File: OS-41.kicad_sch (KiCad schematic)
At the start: 70 parts, among them J1 Conn_01x02_Pin, J2 Conn_01x02_Pin, J3 Conn_01x02_Pin, J4 Conn_Coaxial, J5 Conn_01x02_Pin, J6 Conn_01x04_Pin, J7 Conn_01x09_Pin, J8 Conn_01x02_Pin, J9 Conn_01x02_Pin, U1 GPS1003, U2 SI4432-B1-FMR, U3 MCP1640x-xCHY, U4 ATGM336H-5N31, U5 DS18B20, U6 BMP390L, U7 STM32F411CEUx, X1 SMD-3225_4P 30.000MHZ 10PF, Y1 Crystal_GND24, Y2 Crystal

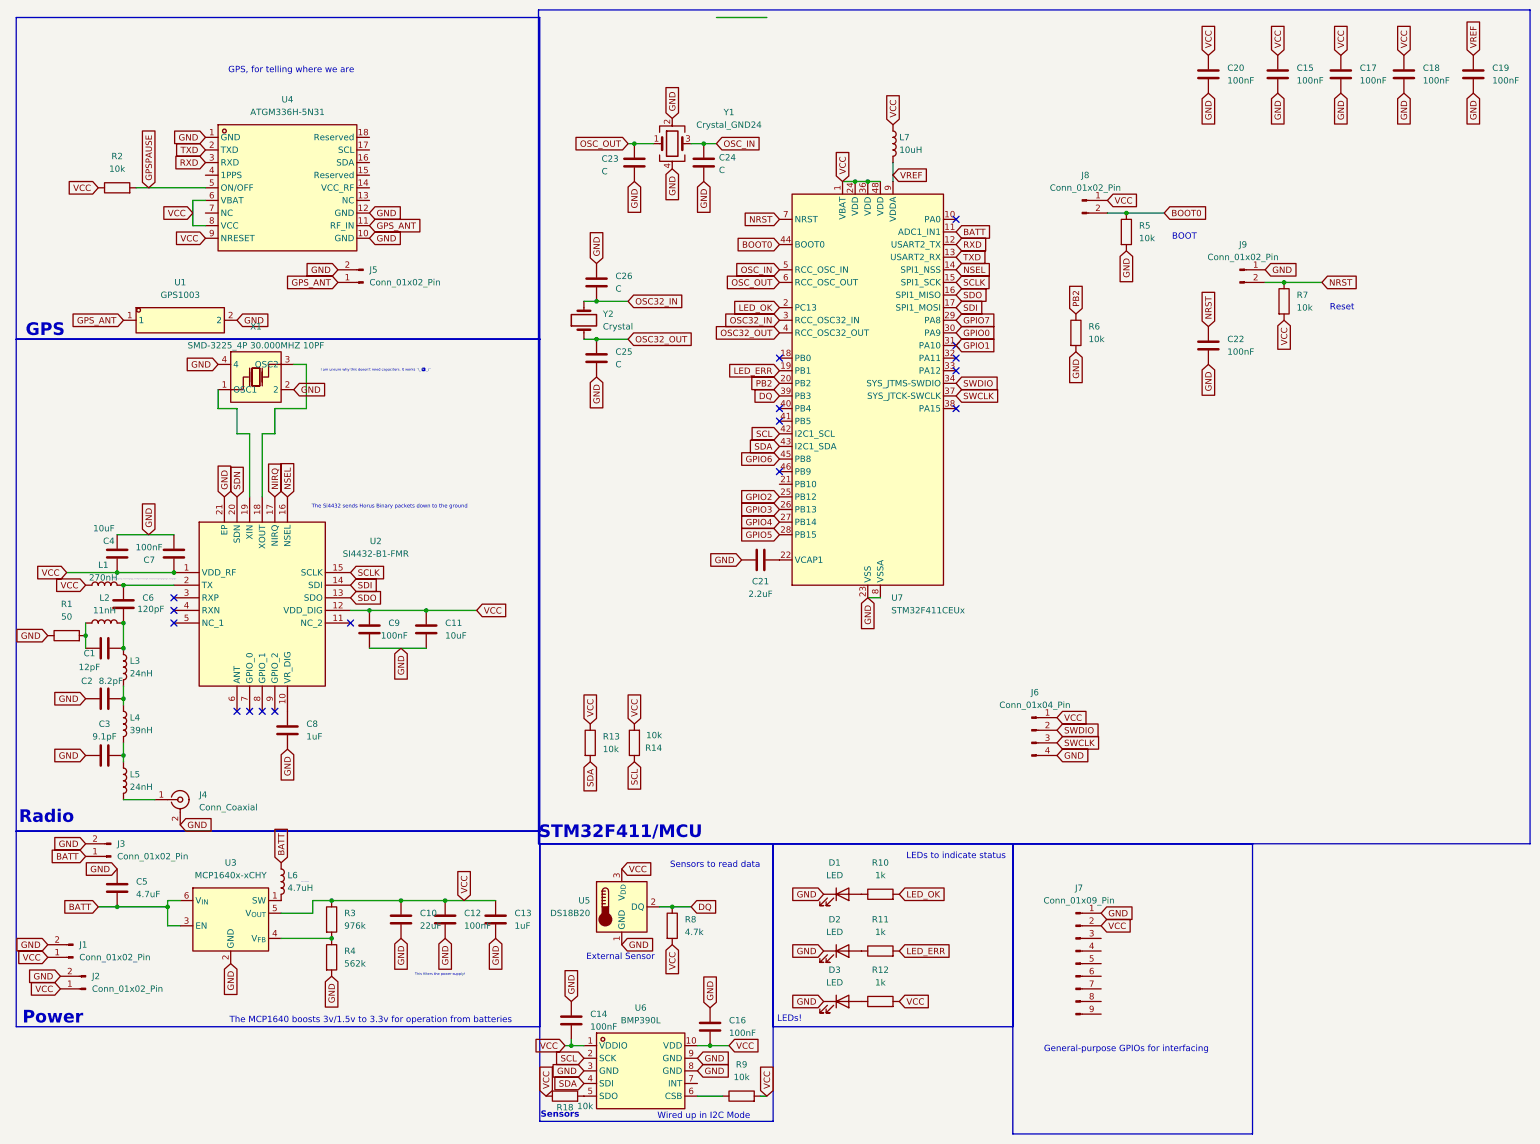
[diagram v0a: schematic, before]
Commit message: Progress
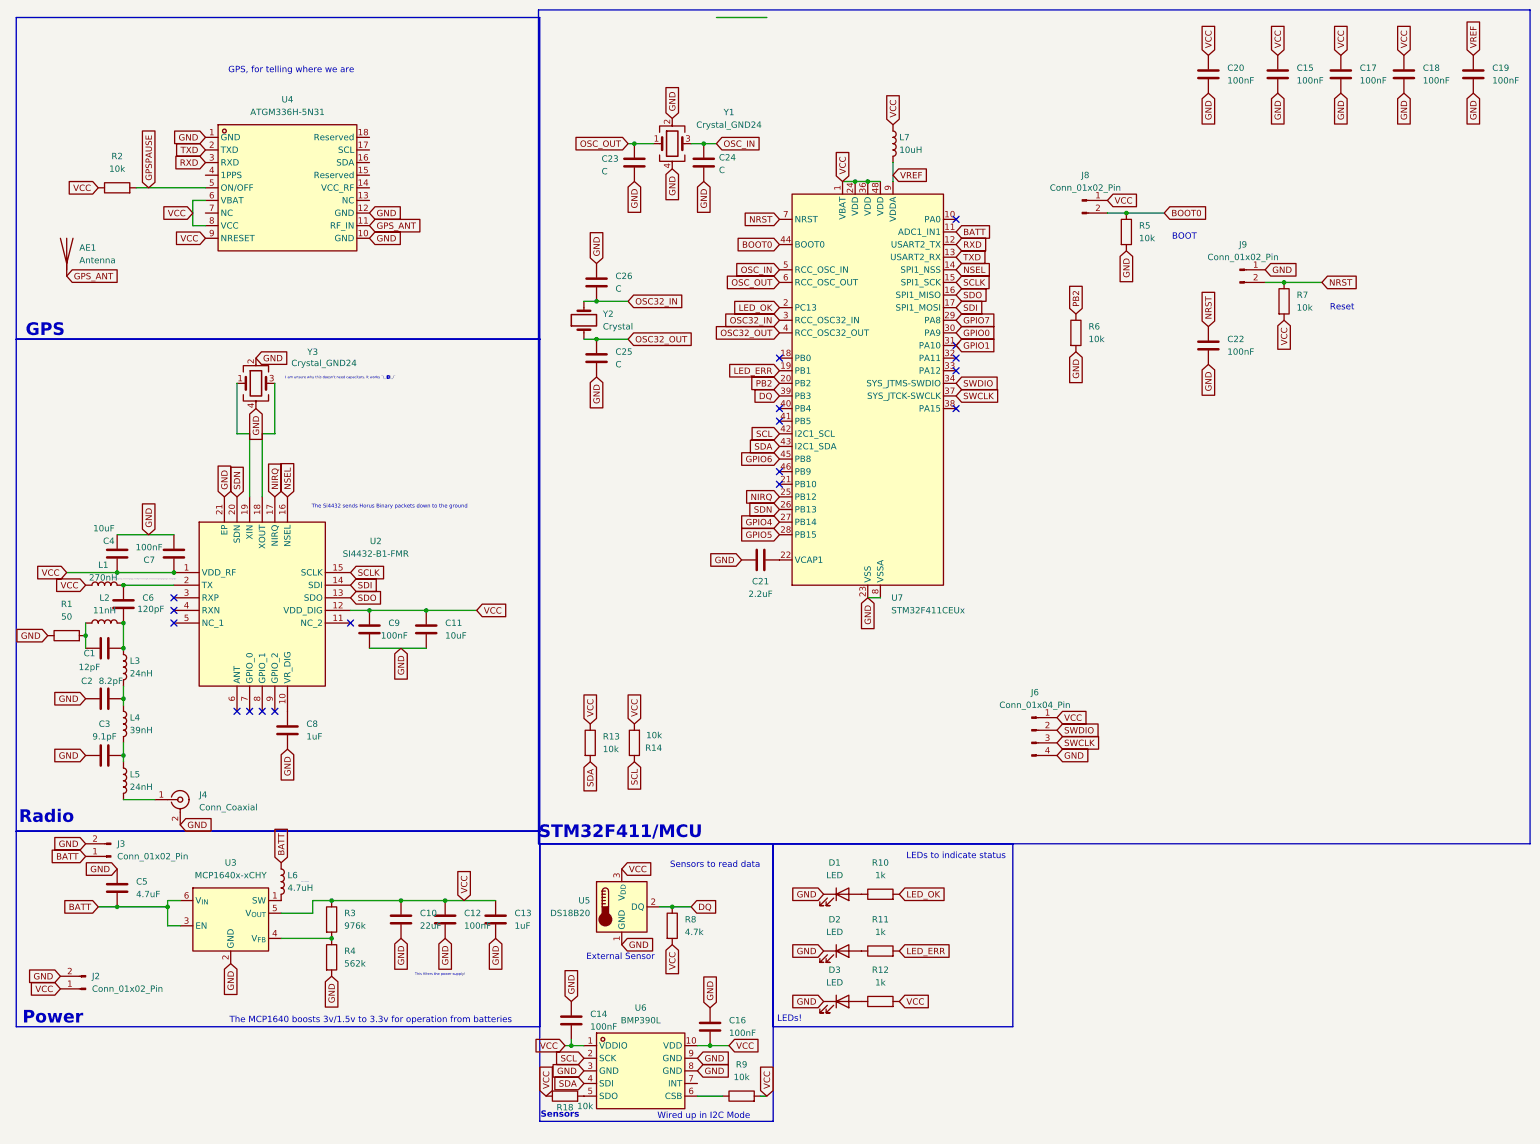
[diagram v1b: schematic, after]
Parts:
- removed J1, J5: Conn_01x02_Pin, Connector_PinSocket_2.54mm:PinSocket_1x02_P2.54mm_Vertical, symbol Connector:Conn_01x02_Pin
- removed J7: Conn_01x09_Pin, Connector_PinSocket_2.54mm:PinSocket_1x09_P2.54mm_Vertical, symbol Connector:Conn_01x09_Pin
- removed U1: GPS1003, libsos41:ANT-SMD_L10.0-W3.0, symbol libs:GPS1003
- removed X1: SMD-3225_4P 30.000MHZ 10PF, libsos41:CRYSTAL-SMD_4P-L3.2-W2.5-BL, symbol crystal:SMD-3225_4P30.000MHZ10PF
- added AE1: Antenna, libsos41:ANT-SMD_L10.0-W3.0, symbol Device:Antenna
- added Y3: Crystal_GND24, Crystal:Crystal_SMD_3225-4Pin_3.2x2.5mm, symbol Device:Crystal_GND24
- C15, C17, C18, C19, C20, C21, C22, C23, C24, C25, C26: footprint (none) -> Capacitor_SMD:C_0603_1608Metric_Pad1.08x0.95mm_HandSolder
- J2, J3: footprint Connector_PinSocket_2.54mm:PinSocket_1x02_P2.54mm_Vertical -> Connector_PinHeader_2.54mm:PinHeader_1x02_P2.54mm_Vertical
- J6: footprint (none) -> Connector_PinHeader_2.54mm:PinHeader_1x04_P2.54mm_Vertical
- J8, J9: footprint (none) -> Connector_PinHeader_2.54mm:PinHeader_1x02_P2.54mm_Vertical
- L7: footprint (none) -> Inductor_SMD:L_0603_1608Metric_Pad1.05x0.95mm_HandSolder
- R5, R6, R7: footprint (none) -> Resistor_SMD:R_0603_1608Metric_Pad0.98x0.95mm_HandSolder
- U2: footprint libsos41:QLP20 -> centdir:QFN50P400X400X90-21N
- Y1: footprint Crystal:Crystal_SMD_3225-4Pin_3.2x2.5mm_HandSoldering -> Crystal:Crystal_SMD_3225-4Pin_3.2x2.5mm
- Y2: footprint (none) -> Crystal:Crystal_SMD_2012-2Pin_2.0x1.2mm_HandSoldering
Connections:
- net GPIO2 is gone; now on net NIRQ: U7.25 (PB12)
- net GPIO3 is gone; now on net SDN: U7.26 (PB13)
- net GND: now also Y3.2, Y3.4
- net GPS_ANT: now also AE1.1 (A)
- net at U2.19 (XIN): now also Y3.1
- net at U2.18 (XOUT): now also Y3.3
- no-connect marks 17 -> 18
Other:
- note removed: "General-purpose GPIOs for interfacing"
